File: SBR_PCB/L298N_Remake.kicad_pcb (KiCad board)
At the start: 2 copper layers, 24 parts, among them J1 Conn_01x02, J2 Conn_01x02, U1 L298N, U2 MPU-6050, U3 AMS1117-3.3, U4 LM7812_TO220

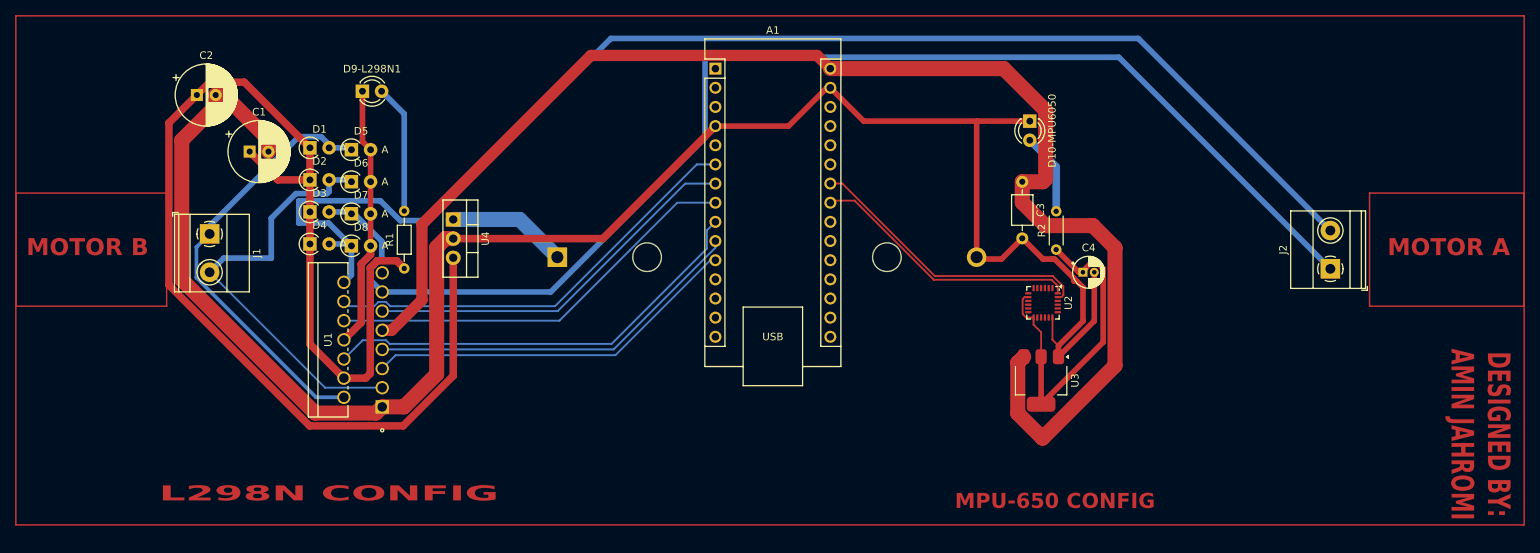
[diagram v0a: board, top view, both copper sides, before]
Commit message: images are added
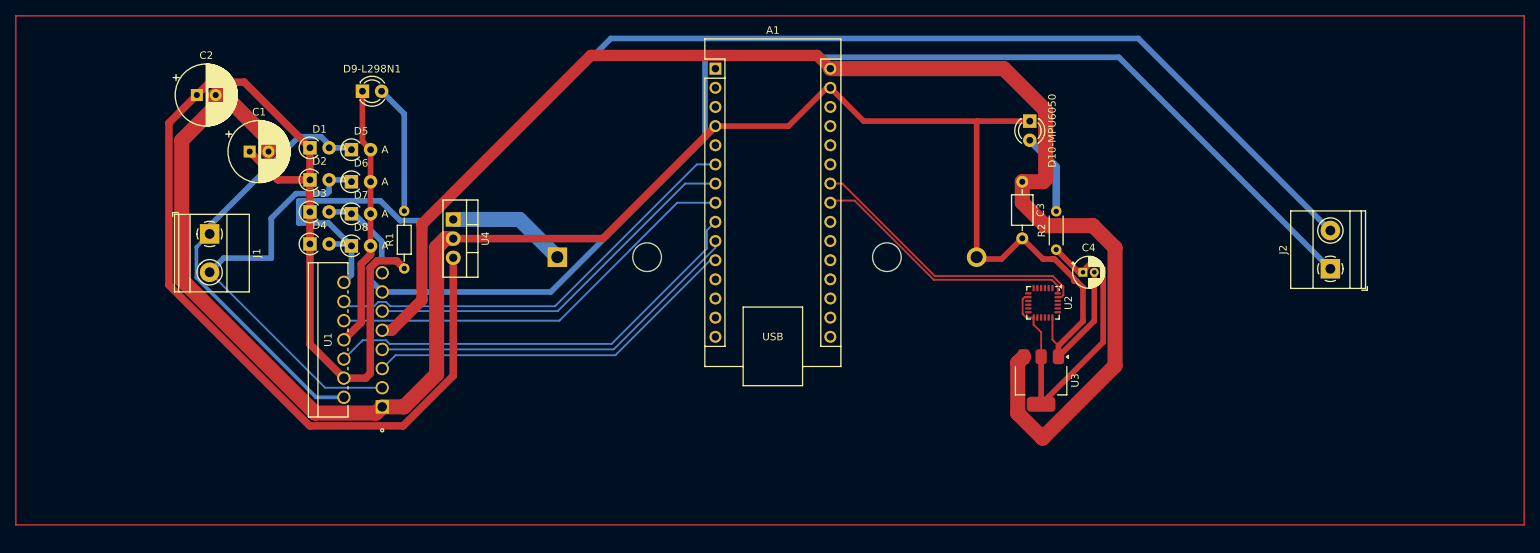
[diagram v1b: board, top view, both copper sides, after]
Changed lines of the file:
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@@
 		)
 		(fp_text user "${REFERENCE}"
-			(at 0 0 360)
+			(at 0 0 0)
 			(layer "F.Fab")
 			(effects
@@
 		(tags "Arduino Nano")
 		(property "Reference" "A1"
-			(at 7.62 -5.08 360)
+			(at 7.62 -5.08 0)
 			(layer "F.SilkS")
 			(effects
@@
 		(tags "CP Radial series Radial pin pitch 1.50mm  diameter 4mm Electrolytic Capacitor")
 		(property "Reference" "C4"
-			(at 0.75 -3.25 360)
+			(at 0.75 -3.25 0)
 			(layer "F.SilkS")
 			(effects
@@
 		)
 		(property "Value" "10µF"
-			(at 0.75 3.25 360)
+			(at 0.75 3.25 0)
 			(layer "F.Fab")
 			(effects
@@
 		)
 		(fp_text user "${REFERENCE}"
-			(at 0.75 0 360)
+			(at 0.75 0 0)
 			(layer "F.Fab")
 			(effects
@@
 		(tags "Bulgin BX0036")
 		(property "Reference" "BT1"
-			(at 27.8 18.1 360)
+			(at 27.8 18.1 0)
 			(layer "B.SilkS")
 			(effects
@@
 		)
 		(property "Value" "Battery"
-			(at 27.8 -1 360)
+			(at 27.8 -1 0)
 			(layer "B.Fab")
 			(effects
@@
 		)
 		(fp_text user "+"
-			(at 3 0.2 360)
+			(at 3 0.2 0)
 			(layer "B.SilkS")
 			(effects
@@
 		)
 		(fp_text user "${REFERENCE}"
-			(at 27.8 1 360)
+			(at 27.8 1 0)
 			(layer "B.Fab")
 			(effects
@@
 	)
 	(gr_rect
-		(start 49 66)
-		(end 69 81)
+		(start 49 42.5)
+		(end 249 110)
 		(stroke
 			(width 0.2)
@@
 	)
 	(gr_rect
-		(start 49 42.5)
-		(end 249 110)
+		(start 49 66)
+		(end 69 81)
 		(stroke
 			(width 0.2)
@@
 		)
 		(fill none)
-		(layer "F.Cu")
-		(net 29)
+		(layer "Dwgs.User")
 	)
 	(gr_rect
@@
 		)
 		(fill none)
-		(layer "F.Cu")
-		(net 29)
+		(layer "Dwgs.User")
 	)
 	(gr_text "DESIGNED BY:\nAMIN JAHROMI"
 		(at 239 98 270)
-		(layer "F.Cu" knockout)
+		(layer "Dwgs.User" knockout)
 		(effects
 			(font
@@
 	(gr_text "MPU-650 CONFIG"
 		(at 173.5 108 0)
-		(layer "F.Cu" knockout)
+		(layer "Dwgs.User" knockout)
 		(effects
 			(font
@@
 	(gr_text "MOTOR A"
 		(at 239 74.5 0)
-		(layer "F.Cu" knockout)
+		(layer "Dwgs.User" knockout)
 		(effects
 			(font
@@
 	(gr_text "MOTOR B"
 		(at 58.5 74.5 0)
-		(layer "F.Cu" knockout)
+		(layer "Dwgs.User" knockout)
 		(effects
 			(font
@@
 	(gr_text "L298N CONFIG"
 		(at 68 107 0)
-		(layer "F.Cu" knockout)
+		(layer "Dwgs.User" knockout)
 		(effects
 			(font
